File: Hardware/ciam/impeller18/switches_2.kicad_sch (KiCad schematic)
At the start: 99 parts, among them J18 430451000, J19 430450800, J20 430450600, J21 430450400, J22 430450600, Q24 BSS138, Q25 BSS138, Q26 BSS138, Q27 BSS138, Q28 BSS138, Q29 BSS138, Q30 BSS138, Q31 BSS138, Q32 BSS138, Q33 BSS138, Q34 BSS138, Q35 BSS138, Q36 BSS138, U26 TLP291-4, U27 TLP291-4, U28 B0505MT-1WR4, U29 TLP291, U30 TLP291, U31 TLP291, U32 TLP291, U33 TLP291

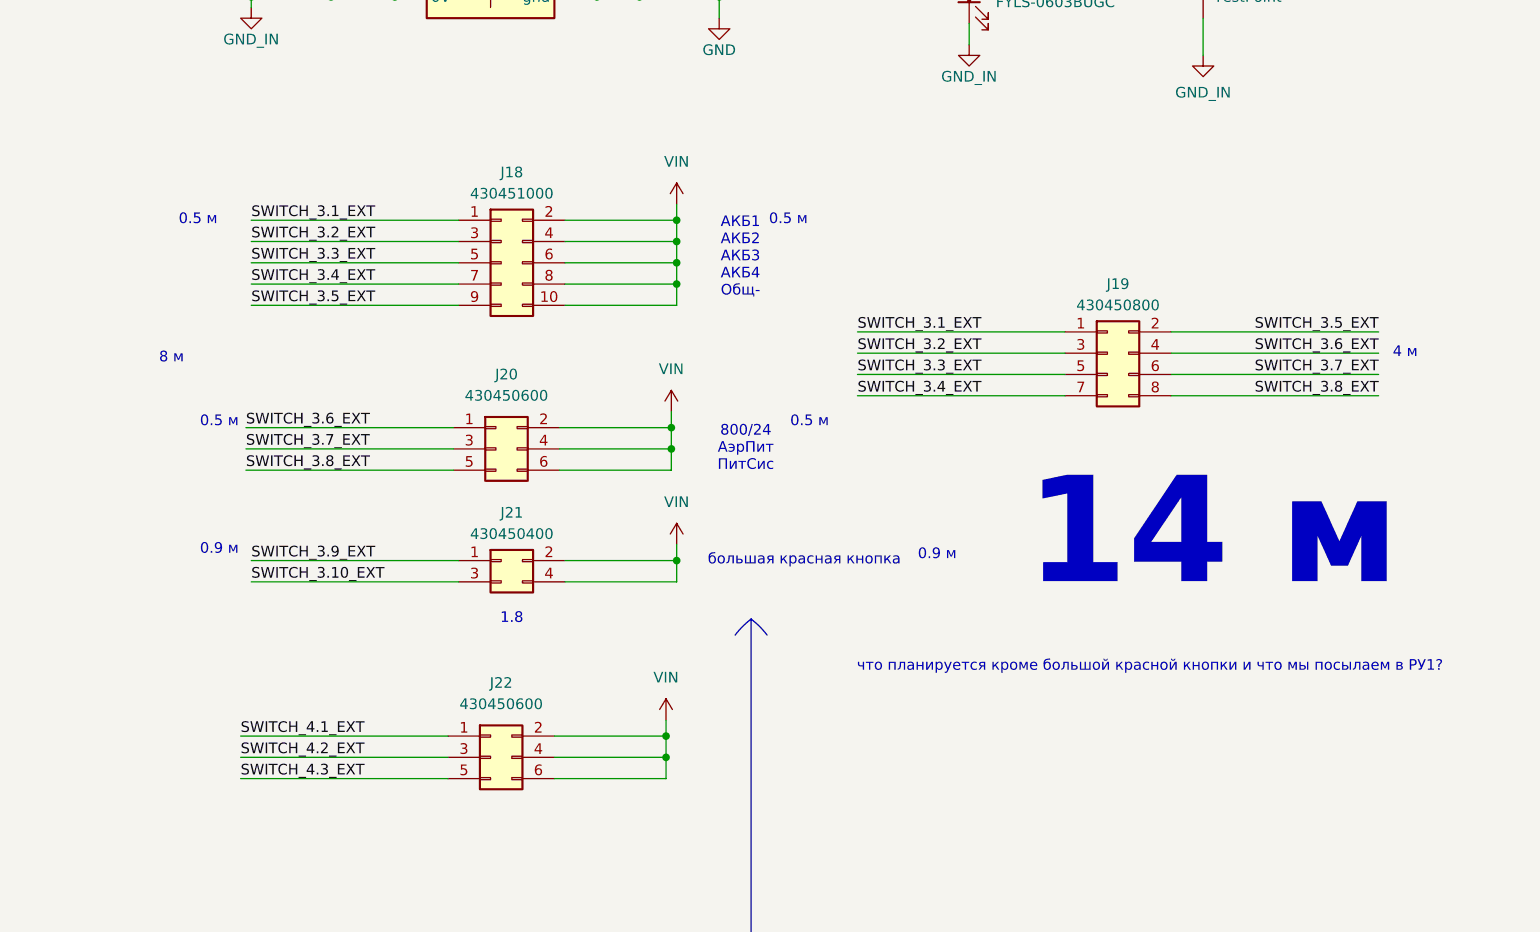
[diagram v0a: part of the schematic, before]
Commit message: Update PCB concept
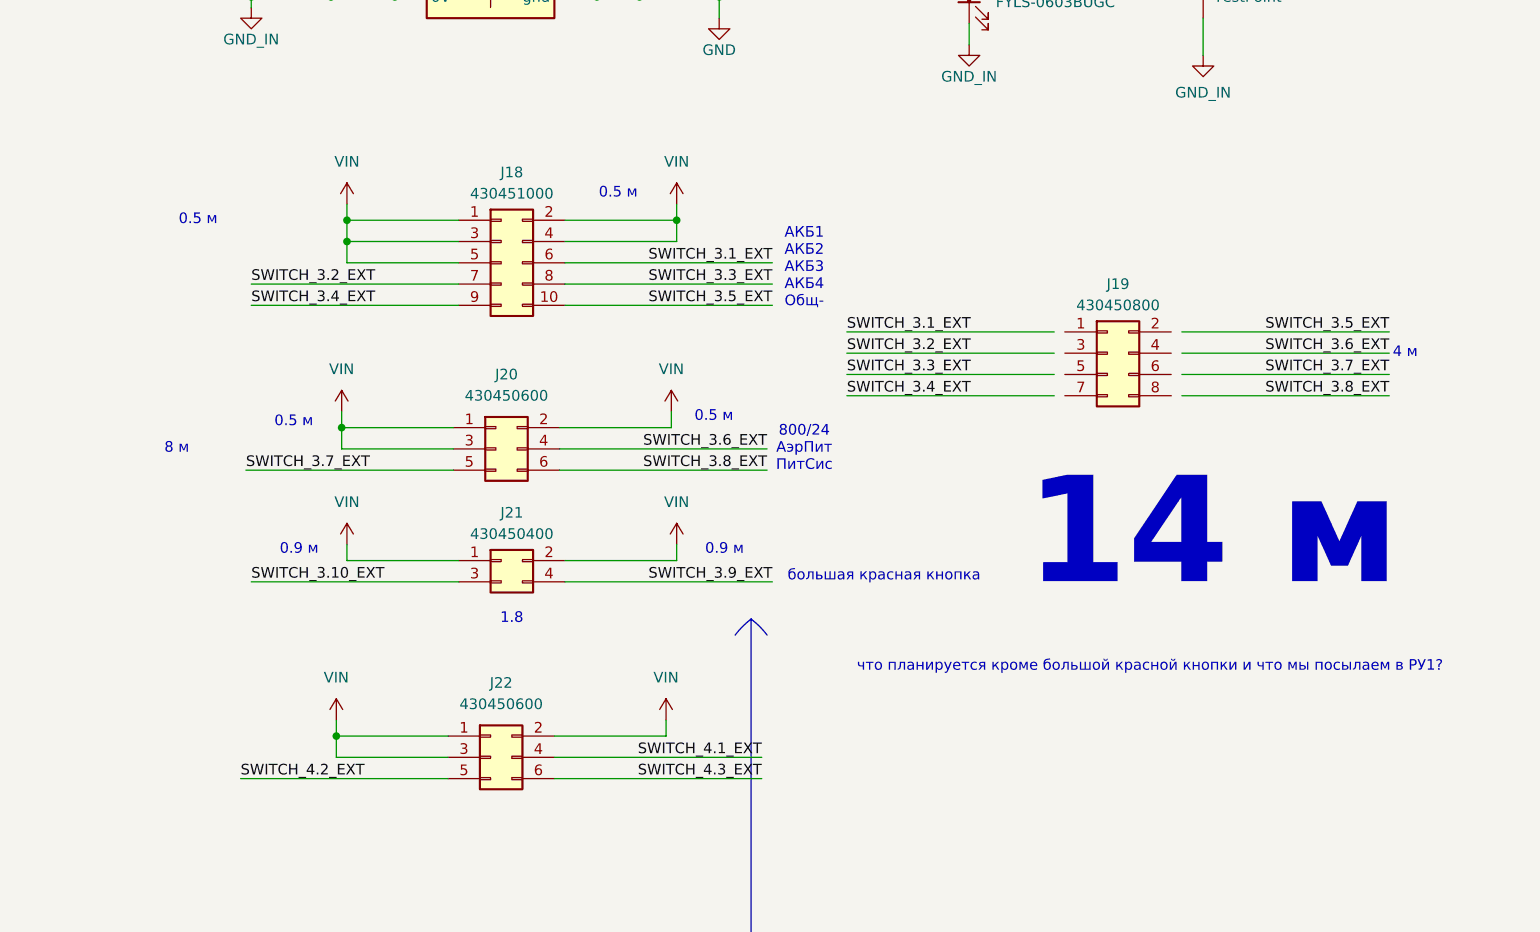
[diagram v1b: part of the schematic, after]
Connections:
- net SWITCH_3.1_EXT: now also J18.6 (Pin_6); no longer J18.1 (Pin_1), J19.1 (Pin_1)
- net SWITCH_3.2_EXT: now also J18.7 (Pin_7); no longer J18.3 (Pin_3), J19.3 (Pin_3)
- net SWITCH_3.3_EXT: now also J18.8 (Pin_8); no longer J18.5 (Pin_5), J19.5 (Pin_5)
- net SWITCH_3.4_EXT: now also J18.9 (Pin_9); no longer J18.7 (Pin_7), J19.7 (Pin_7)
- net SWITCH_3.5_EXT: now also J18.10 (Pin_10); no longer J18.9 (Pin_9), J19.2 (Pin_2)
- net SWITCH_3.6_EXT: now also J20.4 (Pin_4); no longer J19.4 (Pin_4), J20.1 (Pin_1)
- net SWITCH_3.7_EXT: now also J20.5 (Pin_5); no longer J19.6 (Pin_6), J20.3 (Pin_3)
- net SWITCH_3.8_EXT: now also J20.6 (Pin_6); no longer J19.8 (Pin_8), J20.5 (Pin_5)
- net SWITCH_3.9_EXT: now also J21.4 (Pin_4); no longer J21.1 (Pin_1)
- net SWITCH_4.1_EXT: now also J22.4 (Pin_4); no longer J22.1 (Pin_1)
- net SWITCH_4.2_EXT: now also J22.5 (Pin_5); no longer J22.3 (Pin_3)
- net SWITCH_4.3_EXT: now also J22.6 (Pin_6); no longer J22.5 (Pin_5)
- net VIN: now also J18.1 (Pin_1), J18.3 (Pin_3), J18.5 (Pin_5), J20.1 (Pin_1), J20.3 (Pin_3), J21.1 (Pin_1), J22.1 (Pin_1), J22.3 (Pin_3); no longer J18.10 (Pin_10), J18.6 (Pin_6), J18.8 (Pin_8), J20.4 (Pin_4), J20.6 (Pin_6), J21.4 (Pin_4), J22.4 (Pin_4), J22.6 (Pin_6)
